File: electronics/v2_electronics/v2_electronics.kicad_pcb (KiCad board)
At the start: 2 copper layers, 143.5 x 88.9 mm, 45 parts, among them J1 Main Connector, J2 Main Power, J3 12-6V Converter, J4 Controller Battery Connector, J5 Depth Sensor, J6 PinHeader_1x02_P2.54mm_Vertic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, J7 PinHeader_1x08_P2.54mm_Vertic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, J8 PinHeader_1x03_P2.54mm_Vertic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, K1 G5Q-1 5V, K2 G5Q-1 5V, K3 G5Q-1 5V, K4 G5Q-1 5V, K5 T9AS1D12, K6 G5Q-1A 12V, Q1 BC547, Q2 BC547, Q3 BC547, Q4 BC547, Q5 BC547, Q6 BC557, U1 raspberry_pi_pico, U2 mpu6050_breakout

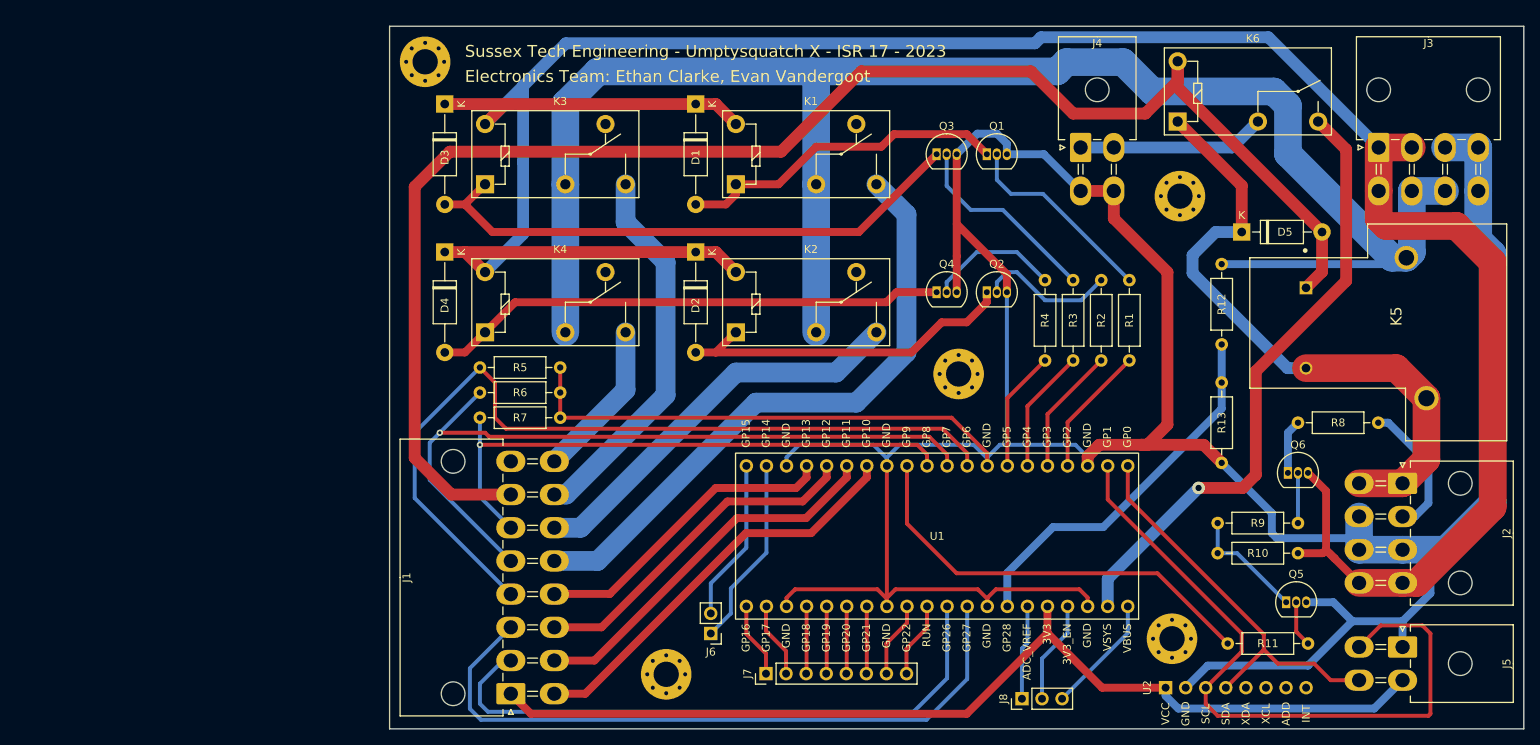
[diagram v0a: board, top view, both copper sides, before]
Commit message: modify pcb and schematic sheets for export for design report
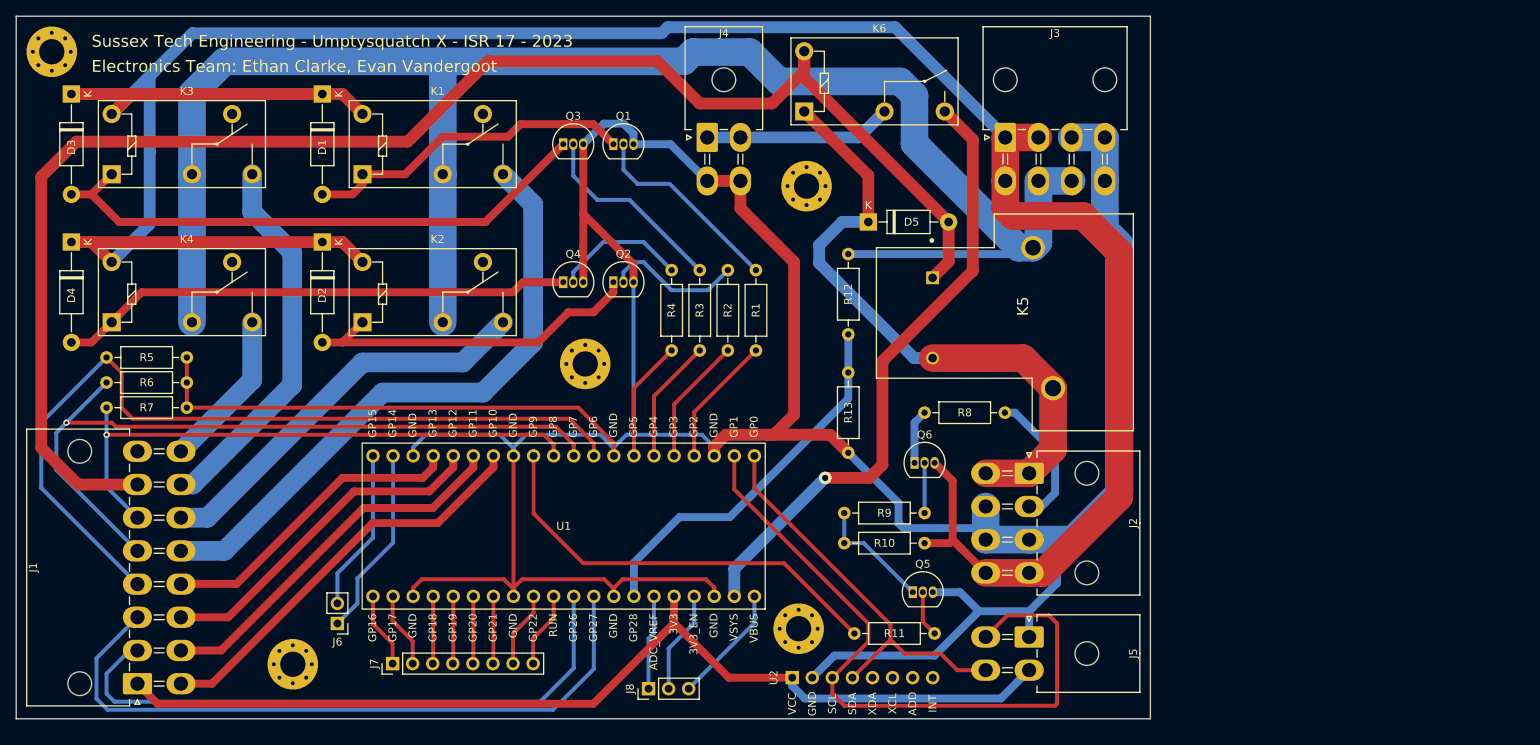
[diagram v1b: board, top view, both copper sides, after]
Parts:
- moved D1 47.3 mm to (109.0, 66.4)
- moved D2 47.3 mm to (109.0, 85.1)
- moved J6 47.3 mm to (110.9, 133.3)
- moved D3 47.3 mm to (77.2, 66.4)
- moved D4 47.3 mm to (77.2, 85.1)
- moved D5 47.3 mm to (178.1, 82.5)
- moved J1 47.3 mm to (85.6, 141.0)
- moved J2 47.3 mm to (198.4, 114.3)
- moved J3 47.3 mm to (195.4, 71.9)
- moved J4 47.3 mm to (157.7, 71.9)
- moved J5 47.3 mm to (198.4, 135.1)
- moved J7 47.3 mm to (117.9, 138.4)
- moved J8 47.3 mm to (150.2, 141.6)
- moved K3 47.3 mm to (82.3, 76.5)
- moved K4 47.3 mm to (82.3, 95.2)
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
